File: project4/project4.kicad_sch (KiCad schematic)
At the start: 22 parts, among them J1 Conn_02x07_Row_Letter_First, J2 Conn_02x07_Row_Letter_First, U1 SST27ST020, U2 SST27ST020, U3 74LS02, U4 74LS670, U5 74LS139, U6 74LS670

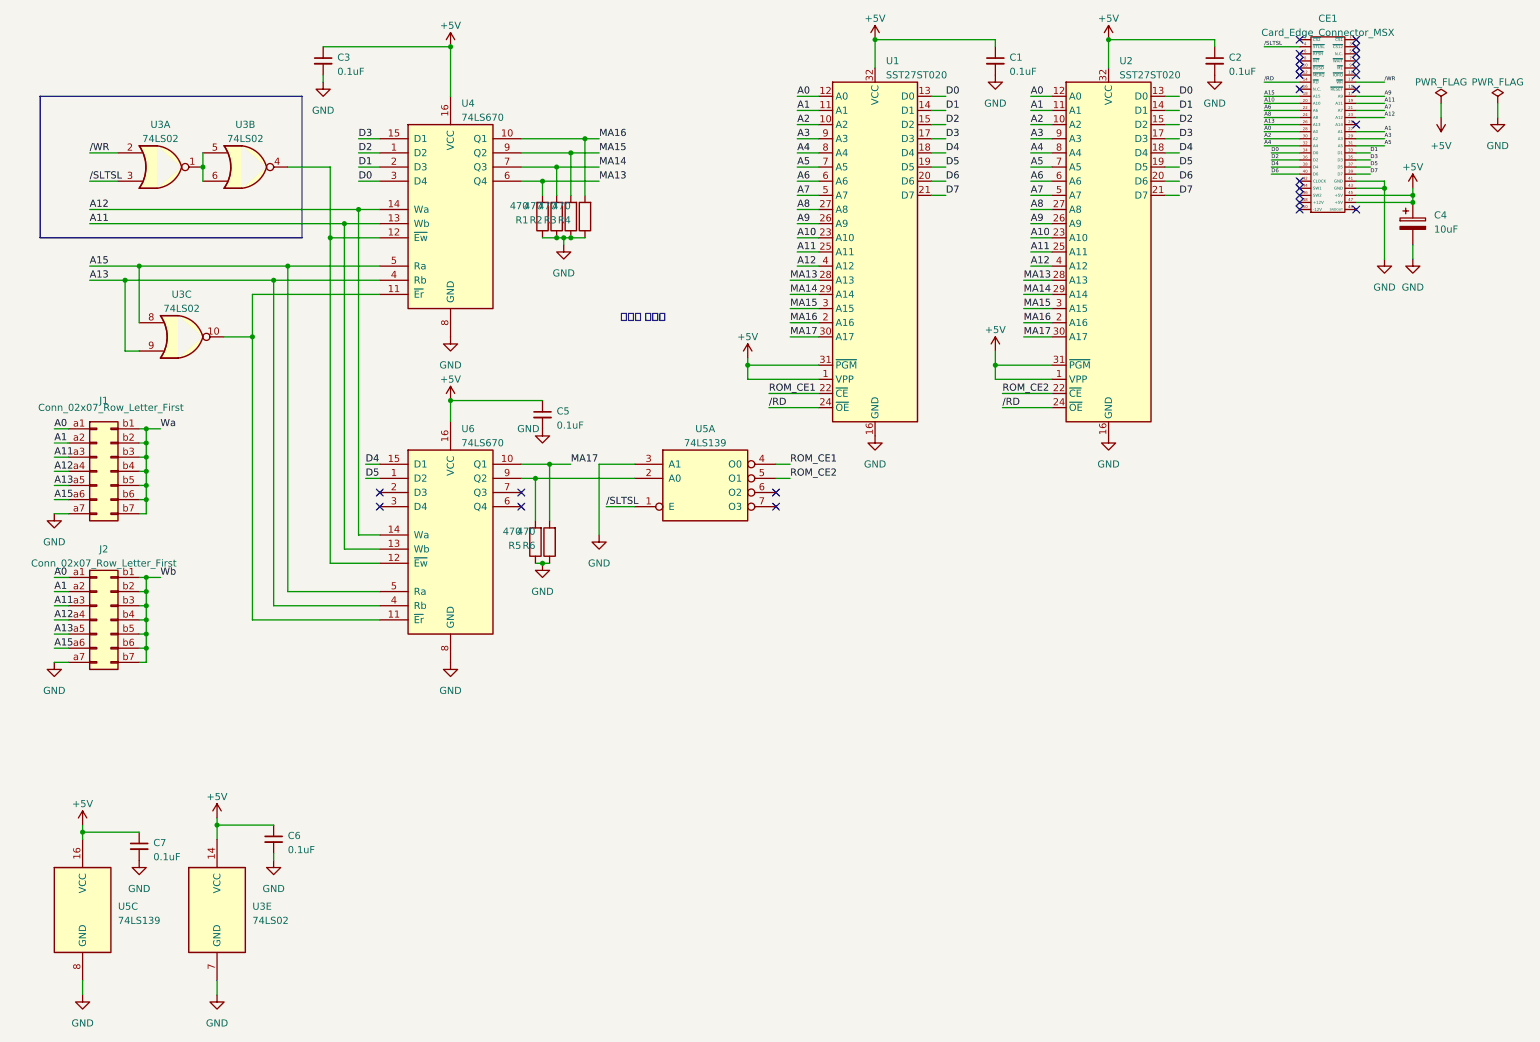
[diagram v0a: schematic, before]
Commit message: Modify project4
Signed-off-by: Youngki Park <ykp7409@gmail.com>
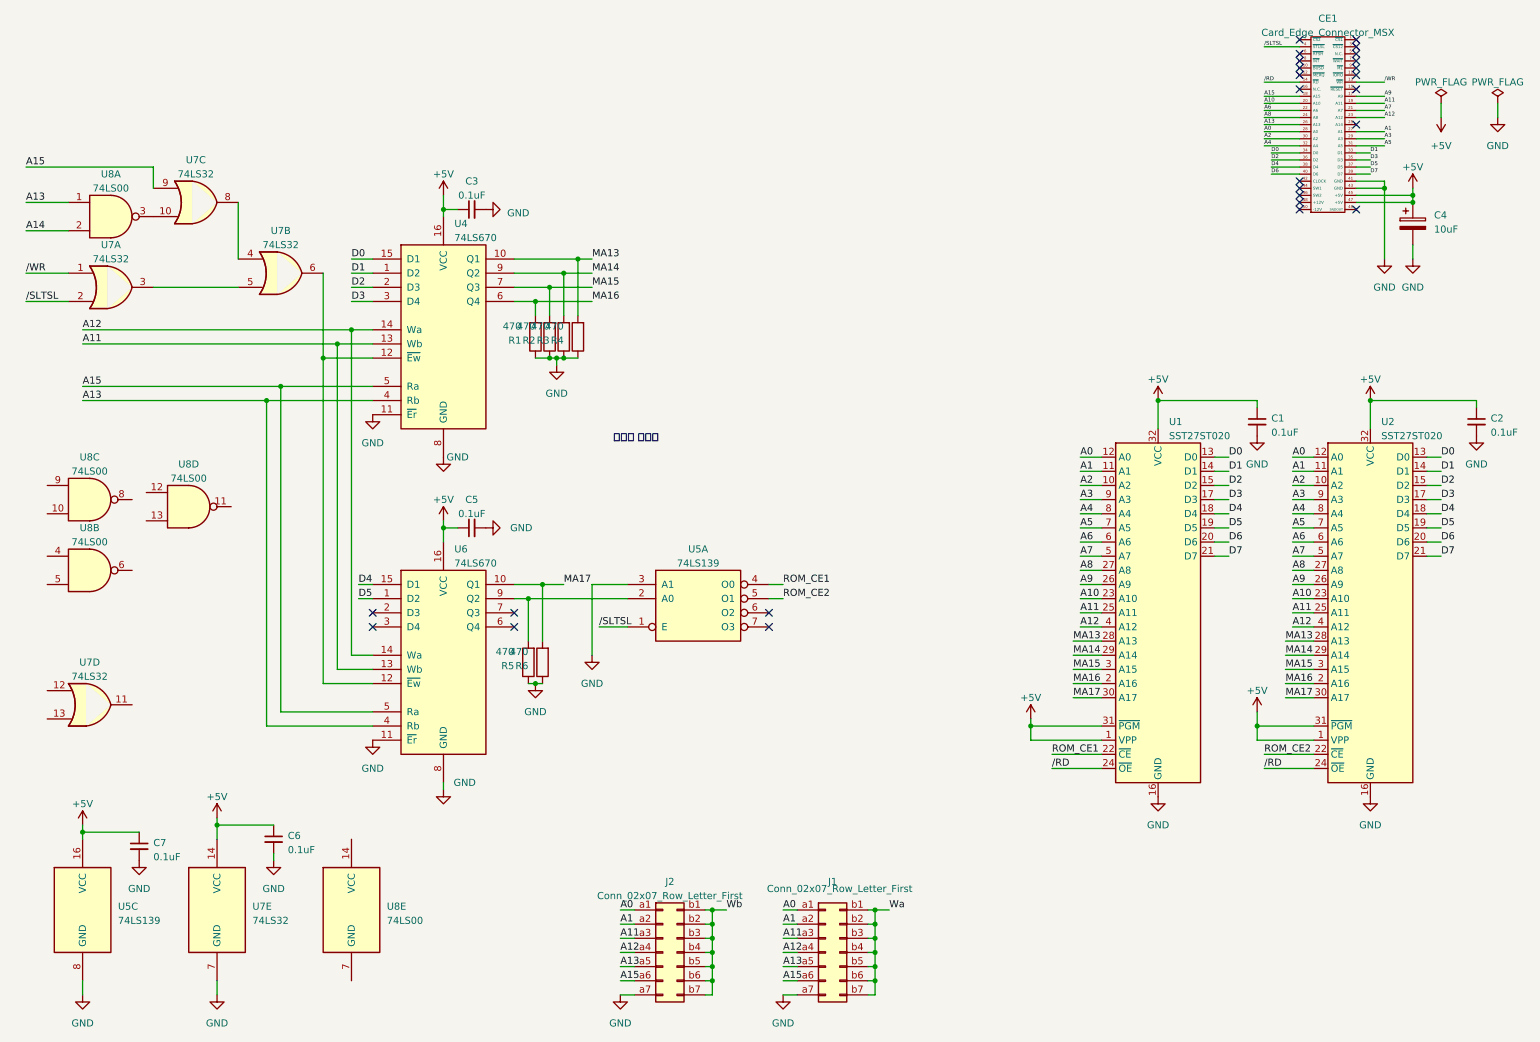
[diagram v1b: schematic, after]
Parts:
- removed U3: 74LS02, Package_DIP:DIP-14_W7.62mm_Socket, symbol 74xx:74LS02
- added U7: 74LS32, symbol 74xx:74LS32
- added U8: 74LS00, symbol 74xx:74LS00
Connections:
- net +5V: now also U7.14 (VCC)
- net A13: now also U8.1
- net A15: now also U7.9
- net D0: now also U4.15 (D1); no longer U4.3 (D4)
- net D1: now also U4.1 (D2); no longer U4.2 (D3)
- net D2: now also U4.2 (D3); no longer U4.1 (D2)
- net D3: now also U4.3 (D4); no longer U4.15 (D1)
- net GND: now also U4.11 (~{Er}), U6.11 (~{Er}), U7.7 (GND)
- net MA13: now also R4.2, U4.10 (Q1); no longer R1.2, U4.6 (Q4)
- net MA14: now also R3.2, U4.9 (Q2); no longer R2.2, U4.7 (Q3)
- net MA15: now also R2.2, U4.7 (Q3); no longer R3.2, U4.9 (Q2)
- net MA16: now also R1.2, U4.6 (Q4); no longer R4.2, U4.10 (Q1)
- net /SLTSL: now also U7.2
- net /WR: now also U7.1
- net at U4.12 (~{Ew}), U6.12 (~{Ew}): now also U7.6
- new net: U7.10, U8.3
- new net: U7.4, U7.8
- new net: U7.3, U7.5
- new net A14: U8.2
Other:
- moved on the sheet: C3, C5, J1, J2, R1, R2, R3, R4, R5, R6, U4, U5A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
